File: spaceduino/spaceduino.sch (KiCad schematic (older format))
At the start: 76 parts, among them J1 USB_B, J3 JICSP, J4 Conn_02x05_Odd_Even, Q1 BSS84, Q2 BSS84, Q3 BSS84, SW1 SW_SPST, U1 TLV70030_SOT23-5, U2 FT230XS, U3 TXB0104D, U4 LM27313XMF, U5 INA226, U6 ATmega1284P-AU, U7 INA226, Y1 Crystal

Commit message: add SD card footprint, PNP-based current mirror
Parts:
- MICROSD1: footprint Spaceduino:HRS_DM3CS-SF -> Spaceduino:Connfly DS1139-06 MicroSD; symbol Connector:Micro_SD_Card_Det -> Connector:Micro_SD_Card; LCSC C202111 -> C86574
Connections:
- net GND: now also J4.1 (Pin_1), J4.9 (Pin_9), MICROSD1.9 (SHIELD); no longer MICROSD1.11 (SHIELD)
- net experiment: now reaches J4.3 (Pin_3)
- net HV-: now reaches J4.5 (Pin_5)
- net HV+: now reaches J4.7 (Pin_7)
- net a3 renamed a3_pump_en
- no-connect marks 15 -> 8
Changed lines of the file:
@@
-	1    0    0    -1
-$EndComp
-$Comp
-L Connector:Micro_SD_Card_Det MICROSD1
-U 1 1 5EFE706C
-P 9600 1650
-F 0 "MICROSD1" H 9550 2467 50  0000 C CNN
-F 1 "Micro_SD_Card_Det" H 9550 2376 50  0000 C CNN
-F 2 "Spaceduino:HRS_DM3CS-SF" H 11650 2350 50  0001 C CNN
-F 3 "https://www.hirose.com/product/en/download_file/key_name/DM3/category/Catalog/doc_file_id/49662/?file_category_id=4&item_id=195&is_series=1" H 9600 1750 50  0001 C CNN
-F 4 "C202111" H 9600 1650 50  0001 C CNN "LCSC"
-	1    9600 1650
 	1    0    0    -1
 $EndComp
 NoConn ~ 8700 1250
 NoConn ~ 8700 1950
-NoConn ~ 8700 2050
-NoConn ~ 8700 2150
 $Comp
 L power:GND #PWR013
@@
 Text Notes 7800 1300 0    50   ~ 0
 The Great Corn Maze
-Wire Wire Line
-	10400 2150 10500 2150
-Wire Wire Line
-	10500 2150 10500 2250
-$Comp
-L power:GND #PWR019
-U 1 1 5EFF3B2C
-P 10500 2250
-F 0 "#PWR019" H 10500 2000 50  0001 C CNN
-F 1 "GND" H 10505 2077 50  0000 C CNN
-F 2 "" H 10500 2250 50  0001 C CNN
-F 3 "" H 10500 2250 50  0001 C CNN
-	1    10500 2250
-	1    0    0    -1
-$EndComp
 Text GLabel 6800 1350 0    50   Input ~ 0
 6_spi_miso
@@
 a2
 Text GLabel 6300 3450 2    50   Input ~ 0
-a3
+a3_pump_en
 Text GLabel 6300 3550 2    50   Input ~ 0
 a4
@@
 $EndComp
 Connection ~ 8300 4850
-NoConn ~ 10050 3350
-NoConn ~ 10050 3450
-NoConn ~ 10050 3550
-NoConn ~ 10050 3650
-NoConn ~ 10050 3750
 $Comp
 L Connector_Generic:Conn_02x05_Odd_Even J4
@@
 Text Notes 1550 6050 1    39   ~ 0
 both blue/white, or zener & led
+Text GLabel 10050 3450 2    50   Input ~ 0
+HV+
+Text GLabel 10050 3550 2    50   Input ~ 0
+HV-
+$Comp
+L power:GND #PWR0115
+U 1 1 6001E502
+P 10050 3750
+F 0 "#PWR0115" H 10050 3500 50  0001 C CNN
+F 1 "GND" H 10055 3577 50  0000 C CNN
+F 2 "" H 10050 3750 50  0001 C CNN
+F 3 "" H 10050 3750 50  0001 C CNN
+	1    10050 3750
+	1    0    0    -1
+$EndComp
+$Comp
+L power:GND #PWR0116
+U 1 1 6001F344
+P 10050 3350
+F 0 "#PWR0116" H 10050 3100 50  0001 C CNN
+F 1 "GND" V 10055 3222 50  0000 R CNN
+F 2 "" H 10050 3350 50  0001 C CNN
+F 3 "" H 10050 3350 50  0001 C CNN
+	1    10050 3350
+	0    -1   -1   0
+$EndComp
+Text GLabel 10050 3650 2    50   Input ~ 0
+experiment
+$Comp
+L power:GND #PWR019
+U 1 1 5EFF3B2C
+P 10500 2250
+F 0 "#PWR019" H 10500 2000 50  0001 C CNN
+F 1 "GND" H 10505 2077 50  0000 C CNN
+F 2 "" H 10500 2250 50  0001 C CNN
+F 3 "" H 10500 2250 50  0001 C CNN
+	1    10500 2250
+	1    0    0    -1
+$EndComp
+Wire Wire Line
+	10500 2150 10500 2250
+Wire Wire Line
+	10400 2150 10500 2150
+$Comp
+L Connector:Micro_SD_Card MICROSD1
+U 1 1 5EFE706C
+P 9600 1550
+F 0 "MICROSD1" H 9550 2367 50  0000 C CNN
+F 1 "Micro_SD_Card_Det" H 9550 2276 50  0000 C CNN
+F 2 "Spaceduino:Connfly DS1139-06 MicroSD" H 11650 2250 50  0001 C CNN
+F 3 "https://datasheet.lcsc.com/szlcsc/CONNFLY-Elec-DS1139-06-08SS4BSR_C86574.pdf" H 9600 1650 50  0001 C CNN
+F 4 "C86574" H 9600 1550 50  0001 C CNN "LCSC"
+	1    9600 1550
+	1    0    0    -1
+$EndComp
 $EndSCHEMATC

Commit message: move more parts to jlcsmt catalog
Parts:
- U5, U7: LCSC (none) -> C49851
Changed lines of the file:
@@
 F 2 "Package_SO:VSSOP-10_3x3mm_P0.5mm" H 9450 5250 50  0001 C CNN
 F 3 "http://www.ti.com/lit/ds/symlink/ina226.pdf" H 9000 5600 50  0001 C CNN
+F 4 "C49851" H 8650 5700 50  0001 C CNN "LCSC"
 	1    8650 5700
 	1    0    0    -1
@@
 F 2 "Package_SO:VSSOP-10_3x3mm_P0.5mm" H 4350 3600 50  0001 C CNN
 F 3 "http://www.ti.com/lit/ds/symlink/ina226.pdf" H 3900 3950 50  0001 C CNN
+F 4 "C49851" H 3550 4050 50  0001 C CNN "LCSC"
 	1    3550 4050
 	1    0    0    -1

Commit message: Added a BJT current mirror using BC846BDW1 NPN BJT's
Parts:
- added Q? (x2): BC846BDW1, Package_TO_SOT_SMD:SOT-363_SC-70-6, symbol Transistor_BJT:BC846BDW1
- added R?: 120, symbol Device:R
- added R?: 3, symbol Device:R
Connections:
- net labels added: V_OUT
- wire segments 179 -> 193
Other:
- moved on the sheet: R17, R18
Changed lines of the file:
@@
 	1    0    0    -1
 $EndComp
-Text GLabel 7700 3050 0    50   Input ~ 0
+Text GLabel 6950 3300 0    50   Input ~ 0
 i2c_scl
 Wire Wire Line
-	7700 3050 7850 3050
-Wire Wire Line
-	7850 3050 7850 2950
+	6950 3300 7100 3300
+Wire Wire Line
+	7100 3300 7100 3200
 $Comp
 L Device:R R17
 U 1 1 5F2124B5
-P 7850 2800
-F 0 "R17" H 7920 2846 50  0000 L CNN
-F 1 "3.3k" H 7920 2755 50  0000 L CNN
-F 2 "Resistor_SMD:R_1206_3216Metric" V 7780 2800 50  0001 C CNN
-F 3 "~" H 7850 2800 50  0001 C CNN
-F 4 "3K3" H 7850 2800 50  0001 C CNN "Comment"
-F 5 "C26032" H 7850 2800 50  0001 C CNN "LCSC"
-	1    7850 2800
+P 7100 3050
+F 0 "R17" H 7170 3096 50  0000 L CNN
+F 1 "3.3k" H 7170 3005 50  0000 L CNN
+F 2 "Resistor_SMD:R_1206_3216Metric" V 7030 3050 50  0001 C CNN
+F 3 "~" H 7100 3050 50  0001 C CNN
+F 4 "3K3" H 7100 3050 50  0001 C CNN "Comment"
+F 5 "C26032" H 7100 3050 50  0001 C CNN "LCSC"
+	1    7100 3050
 	1    0    0    -1
 $EndComp
@@
 L power:+5V #PWR0103
 U 1 1 5F213383
-P 7850 2650
-F 0 "#PWR0103" H 7850 2500 50  0001 C CNN
-F 1 "+5V" H 7865 2823 50  0000 C CNN
-F 2 "" H 7850 2650 50  0001 C CNN
-F 3 "" H 7850 2650 50  0001 C CNN
-	1    7850 2650
-	1    0    0    -1
-$EndComp
-Text GLabel 8350 3050 0    50   Input ~ 0
+P 7100 2900
+F 0 "#PWR0103" H 7100 2750 50  0001 C CNN
+F 1 "+5V" H 7115 3073 50  0000 C CNN
+F 2 "" H 7100 2900 50  0001 C CNN
+F 3 "" H 7100 2900 50  0001 C CNN
+	1    7100 2900
+	1    0    0    -1
+$EndComp
+Text GLabel 7600 3300 0    50   Input ~ 0
 i2c_sda
 Wire Wire Line
-	8350 3050 8500 3050
-Wire Wire Line
-	8500 3050 8500 2950
+	7600 3300 7750 3300
+Wire Wire Line
+	7750 3300 7750 3200
 $Comp
 L Device:R R18
 U 1 1 5F21D6B2
-P 8500 2800
-F 0 "R18" H 8570 2846 50  0000 L CNN
-F 1 "3.3k" H 8570 2755 50  0000 L CNN
-F 2 "Resistor_SMD:R_1206_3216Metric" V 8430 2800 50  0001 C CNN
-F 3 "~" H 8500 2800 50  0001 C CNN
-F 4 "3K3" H 8500 2800 50  0001 C CNN "Comment"
-F 5 "C26032" H 8500 2800 50  0001 C CNN "LCSC"
-	1    8500 2800
+P 7750 3050
+F 0 "R18" H 7820 3096 50  0000 L CNN
+F 1 "3.3k" H 7820 3005 50  0000 L CNN
+F 2 "Resistor_SMD:R_1206_3216Metric" V 7680 3050 50  0001 C CNN
+F 3 "~" H 7750 3050 50  0001 C CNN
+F 4 "3K3" H 7750 3050 50  0001 C CNN "Comment"
+F 5 "C26032" H 7750 3050 50  0001 C CNN "LCSC"
+	1    7750 3050
 	1    0    0    -1
 $EndComp
@@
 L power:+5V #PWR0104
 U 1 1 5F21D6B8
-P 8500 2650
-F 0 "#PWR0104" H 8500 2500 50  0001 C CNN
-F 1 "+5V" H 8515 2823 50  0000 C CNN
-F 2 "" H 8500 2650 50  0001 C CNN
-F 3 "" H 8500 2650 50  0001 C CNN
-	1    8500 2650
+P 7750 2900
+F 0 "#PWR0104" H 7750 2750 50  0001 C CNN
+F 1 "+5V" H 7765 3073 50  0000 C CNN
+F 2 "" H 7750 2900 50  0001 C CNN
+F 3 "" H 7750 2900 50  0001 C CNN
+	1    7750 2900
 	1    0    0    -1
 $EndComp
@@
 $EndComp
 $Sheet
-S 2000 6950 1150 550
+S 1850 6700 1150 550
 U 5F218DF1
 F0 "Custom" 50
@@
 	1    0    0    -1
 $EndComp
+Wire Wire Line
+	8950 3050 9150 3050
+$Comp
+L power:GND #PWR?
+U 1 1 603E39A9
+P 9150 3050
+F 0 "#PWR?" H 9150 2800 50  0001 C CNN
+F 1 "GND" H 9155 2877 50  0000 C CNN
+F 2 "" H 9150 3050 50  0001 C CNN
+F 3 "" H 9150 3050 50  0001 C CNN
+	1    9150 3050
+	1    0    0    -1
+$EndComp
+Connection ~ 9150 3050
+Wire Wire Line
+	9250 2850 9250 2600
+Wire Wire Line
+	9250 2600 8950 2600
+Wire Wire Line
+	8950 2650 8950 2600
+$Comp
+L power:+5V #PWR?
+U 1 1 60433078
+P 8050 2400
+F 0 "#PWR?" H 8050 2250 50  0001 C CNN
+F 1 "+5V" H 8065 2573 50  0000 C CNN
+F 2 "" H 8050 2400 50  0001 C CNN
+F 3 "" H 8050 2400 50  0001 C CNN
+	1    8050 2400
+	1    0    0    -1
+$EndComp
+Wire Wire Line
+	8050 2400 8250 2400
+$Comp
+L Device:R R?
+U 1 1 6043E18A
+P 8700 2400
+F 0 "R?" V 8907 2400 50  0000 C CNN
+F 1 "120" V 8816 2400 50  0000 C CNN
+F 2 "" V 8630 2400 50  0001 C CNN
+F 3 "~" H 8700 2400 50  0001 C CNN
+	1    8700 2400
+	0    -1   -1   0
+$EndComp
+Wire Wire Line
+	8850 2400 8950 2400
+Wire Wire Line
+	8950 2400 8950 2600
+Connection ~ 8950 2600
+Wire Wire Line
+	9550 2650 9550 2400
+Wire Wire Line
+	9550 2400 10150 2400
+Wire Wire Line
+	10150 2400 10150 2700
+Wire Wire Line
+	10150 2700 10400 2700
+Wire Wire Line
+	9150 3050 9550 3050
+$Comp
+L Transistor_BJT:BC846BDW1 Q?
+U 1 1 604D93D7
+P 9450 2850
+F 0 "Q?" H 9640 2896 50  0000 L CNN
+F 1 "BC846BDW1" H 9640 2805 50  0000 L CNN
+F 2 "Package_TO_SOT_SMD:SOT-363_SC-70-6" H 9650 2950 50  0001 C CNN
+F 3 "http://www.onsemi.com/pub_link/Collateral/BC846BDW1T1-D.PDF" H 9450 2850 50  0001 C CNN
+	1    9450 2850
+	1    0    0    -1
+$EndComp
+Connection ~ 9550 3050
+Wire Wire Line
+	9550 3050 10150 3050
+$Comp
+L Transistor_BJT:BC846BDW1 Q?
+U 2 1 604DB938
+P 9050 2850
+F 0 "Q?" H 9241 2896 50  0000 L CNN
+F 1 "BC846BDW1" H 9241 2805 50  0000 L CNN
+F 2 "Package_TO_SOT_SMD:SOT-363_SC-70-6" H 9250 2950 50  0001 C CNN
+F 3 "http://www.onsemi.com/pub_link/Collateral/BC846BDW1T1-D.PDF" H 9050 2850 50  0001 C CNN
+	2    9050 2850
+	-1   0    0    -1
+$EndComp
+Connection ~ 9250 2850
+Wire Wire Line
+	10150 3050 10150 2700
+Connection ~ 10150 2700
+Text GLabel 10400 2700 2    50   Input ~ 0
+V_OUT
+$Comp
+L Device:R R?
+U 1 1 60522A66
+P 8400 2400
+F 0 "R?" V 8607 2400 50  0000 C CNN
+F 1 "3" V 8516 2400 50  0000 C CNN
+F 2 "" V 8330 2400 50  0001 C CNN
+F 3 "~" H 8400 2400 50  0001 C CNN
+	1    8400 2400
+	0    -1   -1   0
+$EndComp
 $EndSCHEMATC

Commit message: Added 500901-0801 Micro SD Socket (locking lid) to schematic, footprint and symbol library, removed current mirror
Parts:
- removed MICROSD1: Micro_SD_Card_Det, Spaceduino:Connfly DS1139-06 MicroSD, symbol Connector:Micro_SD_Card
- removed Q? (x2): BC846BDW1, Package_TO_SOT_SMD:SOT-363_SC-70-6, symbol Transistor_BJT:BC846BDW1
- removed R?: 120, symbol Device:R
- removed R?: 3, symbol Device:R
- added J?: 500901-0801, MOLEX_500901-0801, symbol Spaceduino_Parts:500901-0801
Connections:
- net labels removed: V_OUT
- wire segments 193 -> 177
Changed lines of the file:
@@
 L power:GND #PWR019
 U 1 1 5EFF3B2C
-P 10500 2250
-F 0 "#PWR019" H 10500 2000 50  0001 C CNN
-F 1 "GND" H 10505 2077 50  0000 C CNN
-F 2 "" H 10500 2250 50  0001 C CNN
-F 3 "" H 10500 2250 50  0001 C CNN
-	1    10500 2250
+P 8700 2150
+F 0 "#PWR019" H 8700 1900 50  0001 C CNN
+F 1 "GND" H 8705 1977 50  0000 C CNN
+F 2 "" H 8700 2150 50  0001 C CNN
+F 3 "" H 8700 2150 50  0001 C CNN
+	1    8700 2150
 	1    0    0    -1
 $EndComp
-Wire Wire Line
-	10500 2150 10500 2250
-Wire Wire Line
-	10400 2150 10500 2150
 $Comp
-L Connector:Micro_SD_Card MICROSD1
-U 1 1 5EFE706C
-P 9600 1550
-F 0 "MICROSD1" H 9550 2367 50  0000 C CNN
-F 1 "Micro_SD_Card_Det" H 9550 2276 50  0000 C CNN
-F 2 "Spaceduino:Connfly DS1139-06 MicroSD" H 11650 2250 50  0001 C CNN
-F 3 "https://datasheet.lcsc.com/szlcsc/CONNFLY-Elec-DS1139-06-08SS4BSR_C86574.pdf" H 9600 1650 50  0001 C CNN
-F 4 "C86574" H 9600 1550 50  0001 C CNN "LCSC"
-	1    9600 1550
+L Spaceduino_Parts:500901-0801 J?
+U 1 1 60229AD4
+P 9100 1650
+F 0 "J?" H 9230 1646 50  0000 L CNN
+F 1 "500901-0801" H 9230 1555 50  0000 L CNN
+F 2 "MOLEX_500901-0801" H 9100 1650 50  0001 L BNN
+F 3 "" H 9100 1650 50  0001 L BNN
+F 4 "MOLEX" H 9100 1650 50  0001 L BNN "MANUFACTURER"
+F 5 "MANUFACTURER RECOMMENDATIONS" H 9100 1650 50  0001 L BNN "STANDARD"
+F 6 "H" H 9100 1650 50  0001 L BNN "PART_REV"
+	1    9100 1650
 	1    0    0    -1
 $EndComp
-Wire Wire Line
-	8950 3050 9150 3050
-$Comp
-L power:GND #PWR?
-U 1 1 603E39A9
-P 9150 3050
-F 0 "#PWR?" H 9150 2800 50  0001 C CNN
-F 1 "GND" H 9155 2877 50  0000 C CNN
-F 2 "" H 9150 3050 50  0001 C CNN
-F 3 "" H 9150 3050 50  0001 C CNN
-	1    9150 3050
-	1    0    0    -1
-$EndComp
-Connection ~ 9150 3050
-Wire Wire Line
-	9250 2850 9250 2600
-Wire Wire Line
-	9250 2600 8950 2600
-Wire Wire Line
-	8950 2650 8950 2600
-$Comp
-L power:+5V #PWR?
-U 1 1 60433078
-P 8050 2400
-F 0 "#PWR?" H 8050 2250 50  0001 C CNN
-F 1 "+5V" H 8065 2573 50  0000 C CNN
-F 2 "" H 8050 2400 50  0001 C CNN
-F 3 "" H 8050 2400 50  0001 C CNN
-	1    8050 2400
-	1    0    0    -1
-$EndComp
-Wire Wire Line
-	8050 2400 8250 2400
-$Comp
-L Device:R R?
-U 1 1 6043E18A
-P 8700 2400
-F 0 "R?" V 8907 2400 50  0000 C CNN
-F 1 "120" V 8816 2400 50  0000 C CNN
-F 2 "" V 8630 2400 50  0001 C CNN
-F 3 "~" H 8700 2400 50  0001 C CNN
-	1    8700 2400
-	0    -1   -1   0
-$EndComp
-Wire Wire Line
-	8850 2400 8950 2400
-Wire Wire Line
-	8950 2400 8950 2600
-Connection ~ 8950 2600
-Wire Wire Line
-	9550 2650 9550 2400
-Wire Wire Line
-	9550 2400 10150 2400
-Wire Wire Line
-	10150 2400 10150 2700
-Wire Wire Line
-	10150 2700 10400 2700
-Wire Wire Line
-	9150 3050 9550 3050
-$Comp
-L Transistor_BJT:BC846BDW1 Q?
-U 1 1 604D93D7
-P 9450 2850
-F 0 "Q?" H 9640 2896 50  0000 L CNN
-F 1 "BC846BDW1" H 9640 2805 50  0000 L CNN
-F 2 "Package_TO_SOT_SMD:SOT-363_SC-70-6" H 9650 2950 50  0001 C CNN
-F 3 "http://www.onsemi.com/pub_link/Collateral/BC846BDW1T1-D.PDF" H 9450 2850 50  0001 C CNN
-	1    9450 2850
-	1    0    0    -1
-$EndComp
-Connection ~ 9550 3050
-Wire Wire Line
-	9550 3050 10150 3050
-$Comp
-L Transistor_BJT:BC846BDW1 Q?
-U 2 1 604DB938
-P 9050 2850
-F 0 "Q?" H 9241 2896 50  0000 L CNN
-F 1 "BC846BDW1" H 9241 2805 50  0000 L CNN
-F 2 "Package_TO_SOT_SMD:SOT-363_SC-70-6" H 9250 2950 50  0001 C CNN
-F 3 "http://www.onsemi.com/pub_link/Collateral/BC846BDW1T1-D.PDF" H 9050 2850 50  0001 C CNN
-	2    9050 2850
-	-1   0    0    -1
-$EndComp
-Connection ~ 9250 2850
-Wire Wire Line
-	10150 3050 10150 2700
-Connection ~ 10150 2700
-Text GLabel 10400 2700 2    50   Input ~ 0
-V_OUT
-$Comp
-L Device:R R?
-U 1 1 60522A66
-P 8400 2400
-F 0 "R?" V 8607 2400 50  0000 C CNN
-F 1 "3" V 8516 2400 50  0000 C CNN
-F 2 "" V 8330 2400 50  0001 C CNN
-F 3 "~" H 8400 2400 50  0001 C CNN
-	1    8400 2400
-	0    -1   -1   0
-$EndComp
 $EndSCHEMATC

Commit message: Assigned footprints for SD Card, potentiometer, and resistors
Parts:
- removed J?: 500901-0801, MOLEX_500901-0801, symbol Spaceduino_Parts:500901-0801
- added J2: Micro_SD_Card, Spaceduino:MOLEX_500901-0801, symbol Connector:Micro_SD_Card
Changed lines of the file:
@@
 L power:GND #PWR019
 U 1 1 5EFF3B2C
-P 8700 2150
-F 0 "#PWR019" H 8700 1900 50  0001 C CNN
-F 1 "GND" H 8705 1977 50  0000 C CNN
-F 2 "" H 8700 2150 50  0001 C CNN
-F 3 "" H 8700 2150 50  0001 C CNN
-	1    8700 2150
+P 10400 2150
+F 0 "#PWR019" H 10400 1900 50  0001 C CNN
+F 1 "GND" H 10405 1977 50  0000 C CNN
+F 2 "" H 10400 2150 50  0001 C CNN
+F 3 "" H 10400 2150 50  0001 C CNN
+	1    10400 2150
 	1    0    0    -1
 $EndComp
 $Comp
-L Spaceduino_Parts:500901-0801 J?
-U 1 1 60229AD4
-P 9100 1650
-F 0 "J?" H 9230 1646 50  0000 L CNN
-F 1 "500901-0801" H 9230 1555 50  0000 L CNN
-F 2 "MOLEX_500901-0801" H 9100 1650 50  0001 L BNN
-F 3 "" H 9100 1650 50  0001 L BNN
-F 4 "MOLEX" H 9100 1650 50  0001 L BNN "MANUFACTURER"
-F 5 "MANUFACTURER RECOMMENDATIONS" H 9100 1650 50  0001 L BNN "STANDARD"
-F 6 "H" H 9100 1650 50  0001 L BNN "PART_REV"
-	1    9100 1650
+L Connector:Micro_SD_Card J2
+U 1 1 6025D4E6
+P 9600 1550
+F 0 "J2" H 9550 2267 50  0000 C CNN
+F 1 "Micro_SD_Card" H 9550 2176 50  0000 C CNN
+F 2 "Spaceduino:MOLEX_500901-0801" H 10750 1850 50  0001 C CNN
+F 3 "http://katalog.we-online.de/em/datasheet/693072010801.pdf" H 9600 1550 50  0001 C CNN
+	1    9600 1550
 	1    0    0    -1
 $EndComp

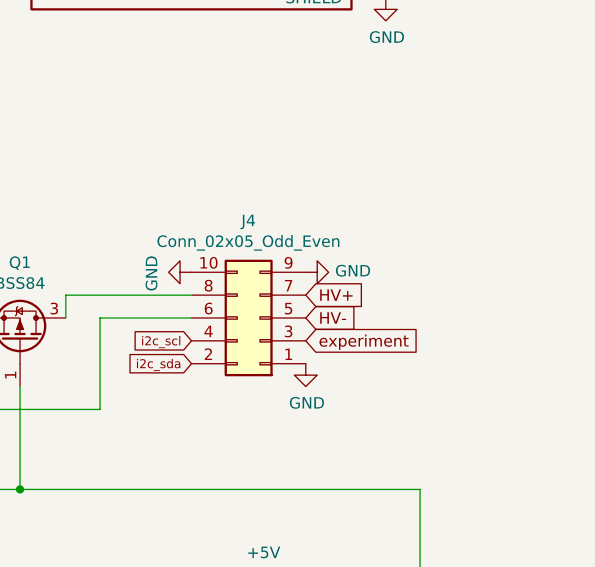
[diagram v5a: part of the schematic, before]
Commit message: inner containment baord lookin pretty good
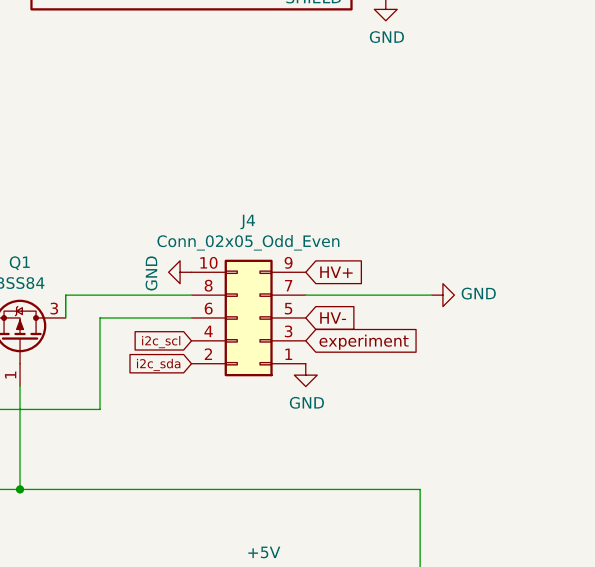
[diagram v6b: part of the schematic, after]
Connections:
- net GND: now also J4.7 (Pin_7); no longer J4.9 (Pin_9)
- net HV+: now also J4.9 (Pin_9); no longer J4.7 (Pin_7)
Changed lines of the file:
@@
 Text Notes 1550 6050 1    39   ~ 0
 both blue/white, or zener & led
-Text GLabel 10050 3450 2    50   Input ~ 0
+Text GLabel 10050 3350 2    50   Input ~ 0
 HV+
 Text GLabel 10050 3550 2    50   Input ~ 0
@@
 	1    0    0    -1
 $EndComp
-$Comp
-L power:GND #PWR0116
-U 1 1 6001F344
-P 10050 3350
-F 0 "#PWR0116" H 10050 3100 50  0001 C CNN
-F 1 "GND" V 10055 3222 50  0000 R CNN
-F 2 "" H 10050 3350 50  0001 C CNN
-F 3 "" H 10050 3350 50  0001 C CNN
-	1    10050 3350
-	0    -1   -1   0
-$EndComp
-Text GLabel 10050 3650 2    50   Input ~ 0
-experiment
 $Comp
 L power:GND #PWR019
@@
 	1    0    0    -1
 $EndComp
+Text GLabel 10050 3650 2    50   Input ~ 0
+experiment
+Wire Wire Line
+	10050 3450 10600 3450
+$Comp
+L power:GND #PWR?
+U 1 1 60543884
+P 10600 3450
+F 0 "#PWR?" H 10600 3200 50  0001 C CNN
+F 1 "GND" V 10605 3322 50  0000 R CNN
+F 2 "" H 10600 3450 50  0001 C CNN
+F 3 "" H 10600 3450 50  0001 C CNN
+	1    10600 3450
+	0    -1   -1   0
+$EndComp
 $EndSCHEMATC

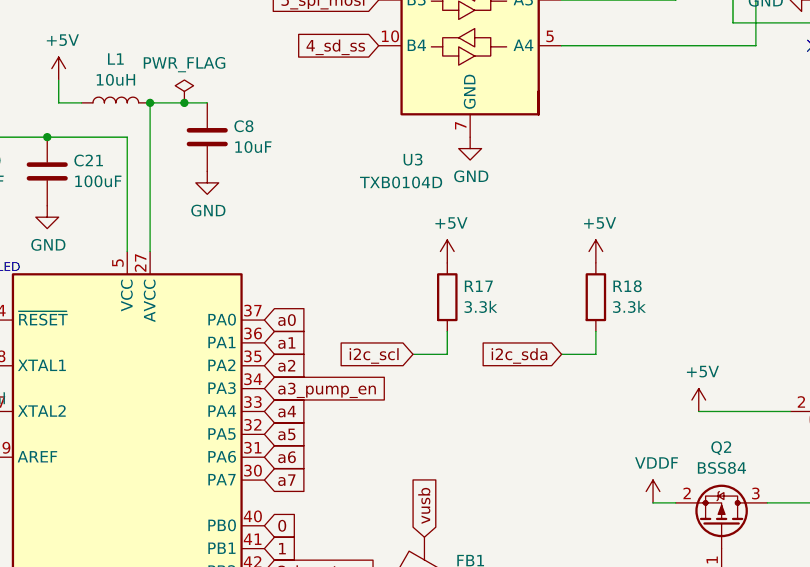
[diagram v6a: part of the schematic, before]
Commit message: spaceduino laid out???
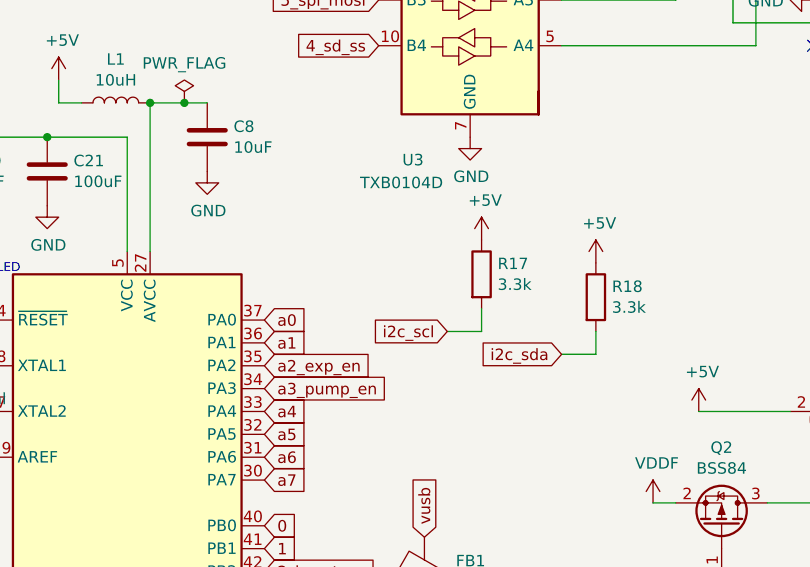
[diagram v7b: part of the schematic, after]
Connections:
- net a2 renamed a2_exp_en
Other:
- moved on the sheet: R17
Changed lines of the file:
@@
 a1
 Text GLabel 6300 3350 2    50   Input ~ 0
-a2
+a2_exp_en
 Text GLabel 6300 3450 2    50   Input ~ 0
 a3_pump_en
@@
 	1    0    0    -1
 $EndComp
-Text GLabel 6950 3300 0    50   Input ~ 0
+Text GLabel 7100 3200 0    50   Input ~ 0
 i2c_scl
 Wire Wire Line
-	6950 3300 7100 3300
-Wire Wire Line
-	7100 3300 7100 3200
+	7100 3200 7250 3200
+Wire Wire Line
+	7250 3200 7250 3100
 $Comp
 L Device:R R17
 U 1 1 5F2124B5
-P 7100 3050
-F 0 "R17" H 7170 3096 50  0000 L CNN
-F 1 "3.3k" H 7170 3005 50  0000 L CNN
-F 2 "Resistor_SMD:R_1206_3216Metric" V 7030 3050 50  0001 C CNN
-F 3 "~" H 7100 3050 50  0001 C CNN
-F 4 "3K3" H 7100 3050 50  0001 C CNN "Comment"
-F 5 "C26032" H 7100 3050 50  0001 C CNN "LCSC"
-	1    7100 3050
+P 7250 2950
+F 0 "R17" H 7320 2996 50  0000 L CNN
+F 1 "3.3k" H 7320 2905 50  0000 L CNN
+F 2 "Resistor_SMD:R_1206_3216Metric" V 7180 2950 50  0001 C CNN
+F 3 "~" H 7250 2950 50  0001 C CNN
+F 4 "3K3" H 7250 2950 50  0001 C CNN "Comment"
+F 5 "C26032" H 7250 2950 50  0001 C CNN "LCSC"
+	1    7250 2950
 	1    0    0    -1
 $EndComp
@@
 L power:+5V #PWR0103
 U 1 1 5F213383
-P 7100 2900
-F 0 "#PWR0103" H 7100 2750 50  0001 C CNN
-F 1 "+5V" H 7115 3073 50  0000 C CNN
-F 2 "" H 7100 2900 50  0001 C CNN
-F 3 "" H 7100 2900 50  0001 C CNN
-	1    7100 2900
+P 7250 2800
+F 0 "#PWR0103" H 7250 2650 50  0001 C CNN
+F 1 "+5V" H 7265 2973 50  0000 C CNN
+F 2 "" H 7250 2800 50  0001 C CNN
+F 3 "" H 7250 2800 50  0001 C CNN
+	1    7250 2800
 	1    0    0    -1
 $EndComp
@@
 	10050 3450 10600 3450
 $Comp
-L power:GND #PWR?
+L power:GND #PWR0116
 U 1 1 60543884
 P 10600 3450
-F 0 "#PWR?" H 10600 3200 50  0001 C CNN
+F 0 "#PWR0116" H 10600 3200 50  0001 C CNN
 F 1 "GND" V 10605 3322 50  0000 R CNN
 F 2 "" H 10600 3450 50  0001 C CNN

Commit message: use sd card that is actually in stock on digikey
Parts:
- J2: footprint Spaceduino:MOLEX_500901-0801 -> Spaceduino:HRS_DM3CS-SF
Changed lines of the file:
@@
 F 0 "J2" H 9550 2267 50  0000 C CNN
 F 1 "Micro_SD_Card" H 9550 2176 50  0000 C CNN
-F 2 "Spaceduino:MOLEX_500901-0801" H 10750 1850 50  0001 C CNN
+F 2 "Spaceduino:HRS_DM3CS-SF" H 10750 1850 50  0001 C CNN
 F 3 "http://katalog.we-online.de/em/datasheet/693072010801.pdf" H 9600 1550 50  0001 C CNN
 	1    9600 1550
